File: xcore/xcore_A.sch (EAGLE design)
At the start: 40 parts, among them U1 NC7WZ07, X1 XEF216-512-TQ128

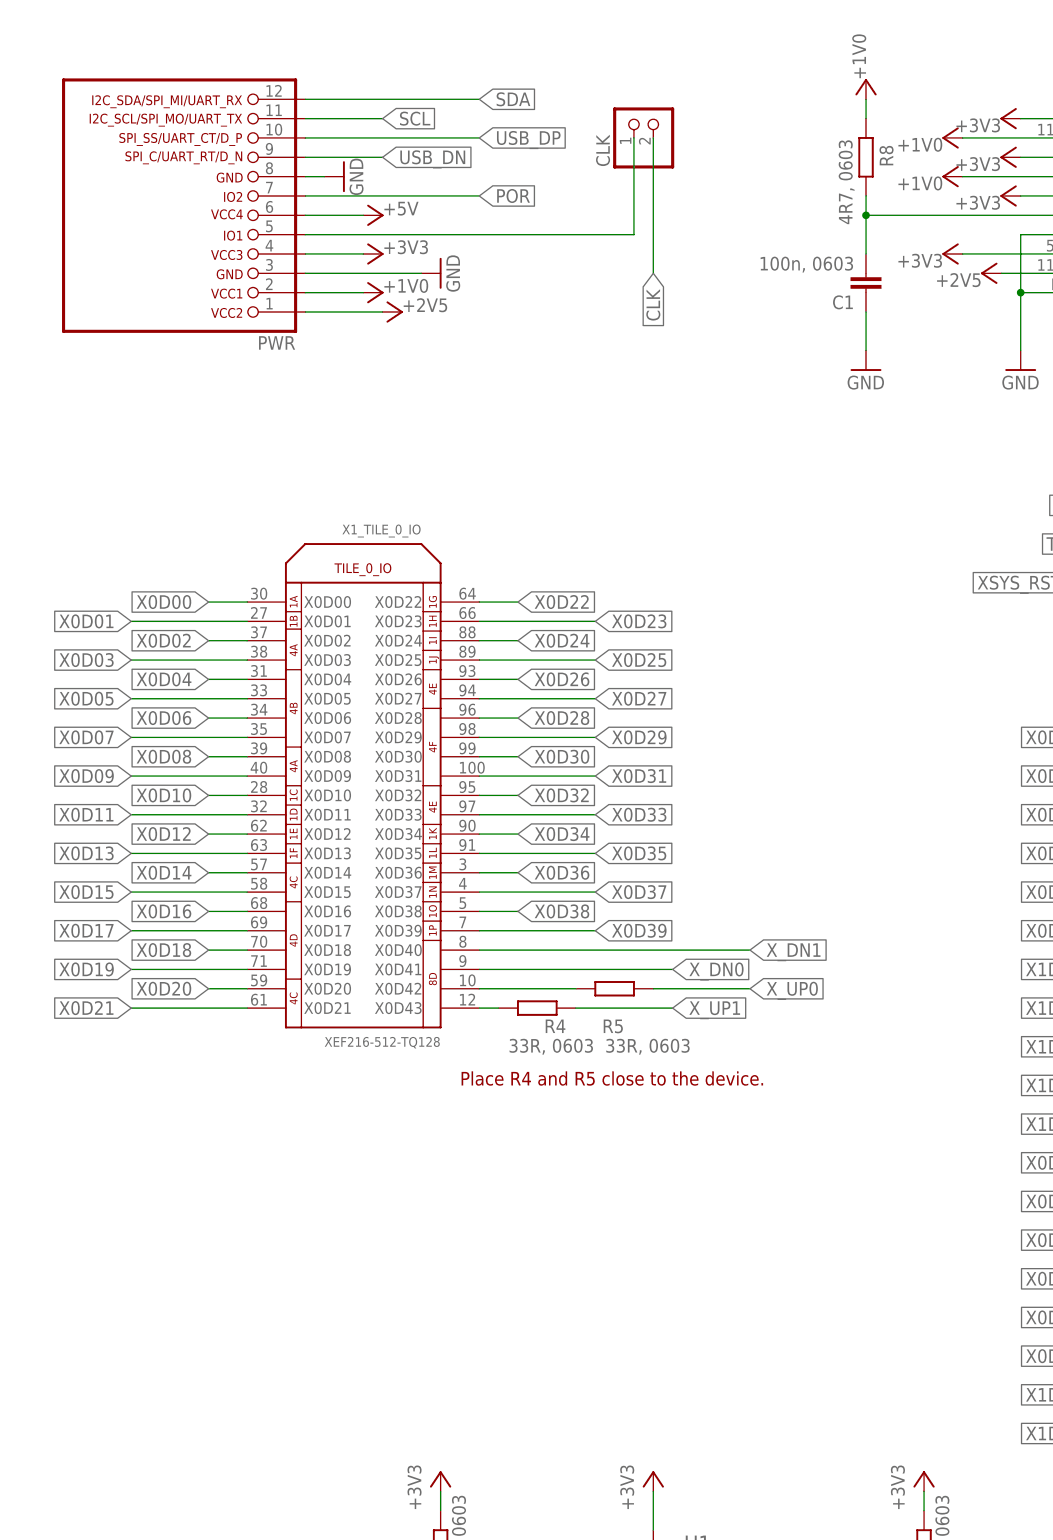
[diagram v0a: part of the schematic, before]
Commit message: xcore: updated with liwe 40 8x8 device
Signed-off-by: malo <pavol.malosek@gmail.com>
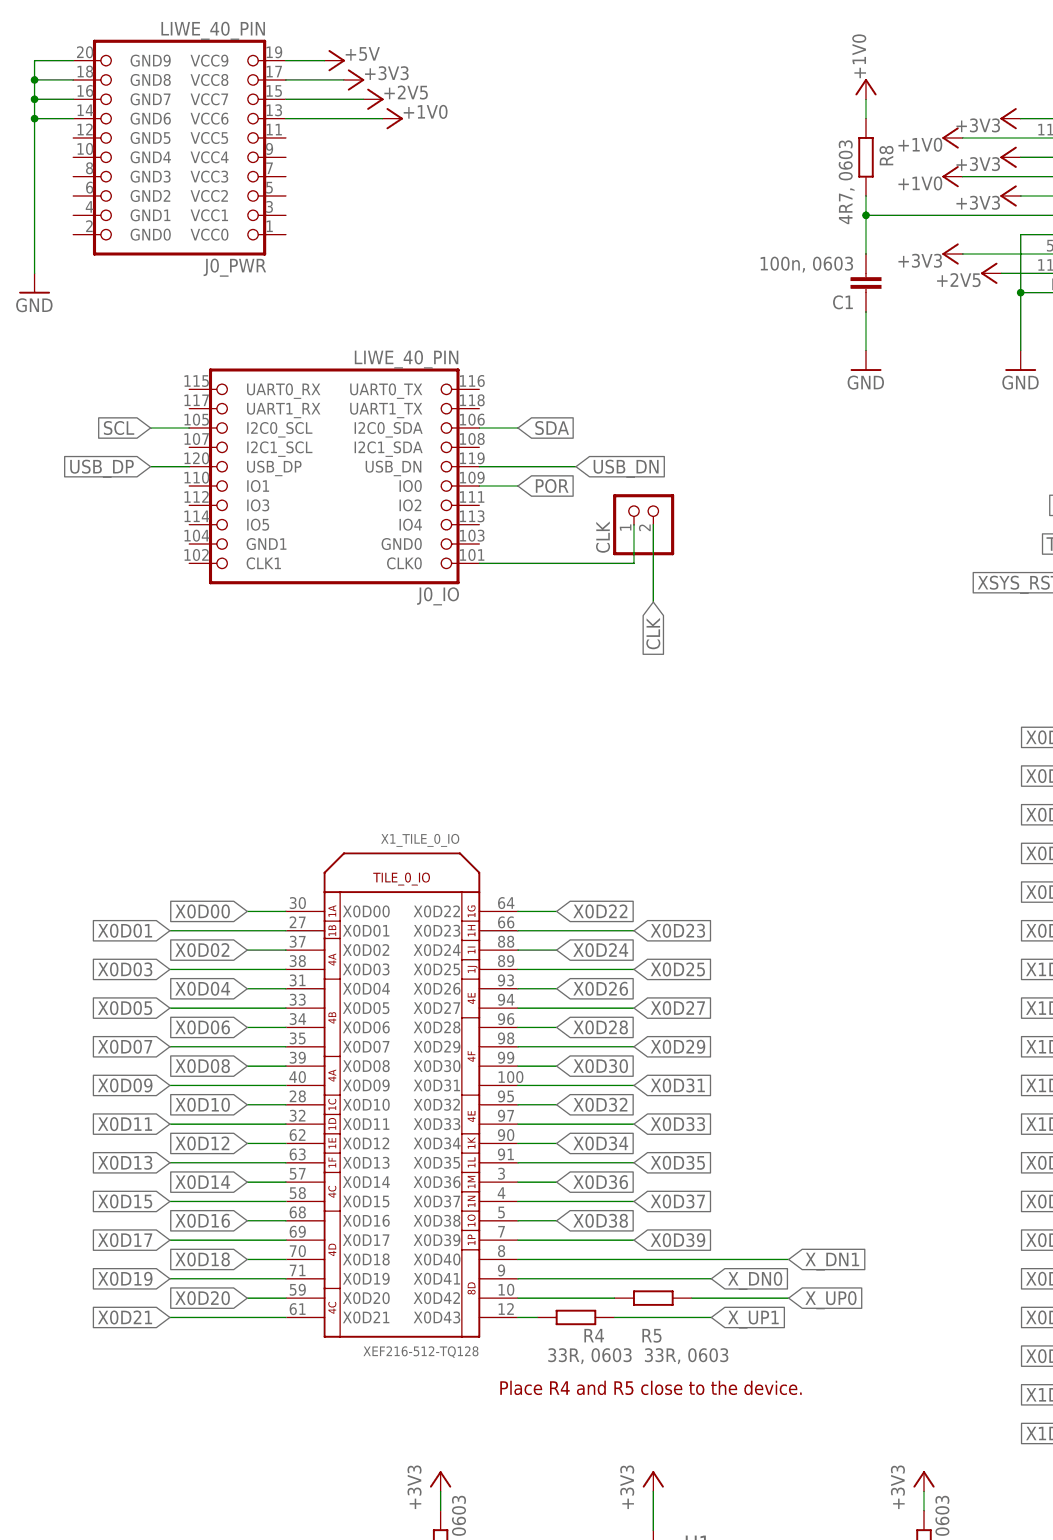
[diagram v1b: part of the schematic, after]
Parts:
- removed PWR: (no value), 25cmsquare:LIWE_12_PIN_PWR8X8_COMPAT
- added J0: LIWE_40_PIN, 25cmsquare:LIWE_40_PIN
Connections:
- net +1V0: now also J0_PWR.VCC6; no longer PWR.2
- net +2V5: now also J0_PWR.VCC7; no longer PWR.1
- net +3V3: now also J0_PWR.VCC8; no longer PWR.4
- net +5V: now also J0_PWR.VCC9; no longer PWR.6
- net GND: now also J0_PWR.GND6, J0_PWR.GND7, J0_PWR.GND8, J0_PWR.GND9; no longer PWR.3, PWR.8
- net IO1: now also J0_IO.CLK0; no longer PWR.5
- net POR: now also J0_IO.IO0; no longer PWR.7
- net SCL: now also J0_IO.I2C0_SCL; no longer PWR.11
- net SDA: now also J0_IO.I2C0_SDA; no longer PWR.12
- net USB_DN: now also J0_IO.USB_DN; no longer PWR.9
- net USB_DP: now also J0_IO.USB_DP; no longer PWR.10
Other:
- moved on the sheet: CLK, R4, R5, X1_TILE_0_IO
